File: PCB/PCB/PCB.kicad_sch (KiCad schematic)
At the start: 30 parts, among them J1 AudioJack Right, J2 USB_B_Micro, J3 AudioJack Left, Q1 BC817, Q2 BC817, Q3 BSS84, U1 ESP32-S3-WROOM-1, U2 CP2102N-Axx-xQFN28, U3 NCP1117-3.3_SOT223, U4 UDA1334ATS, U5 PAM8403D

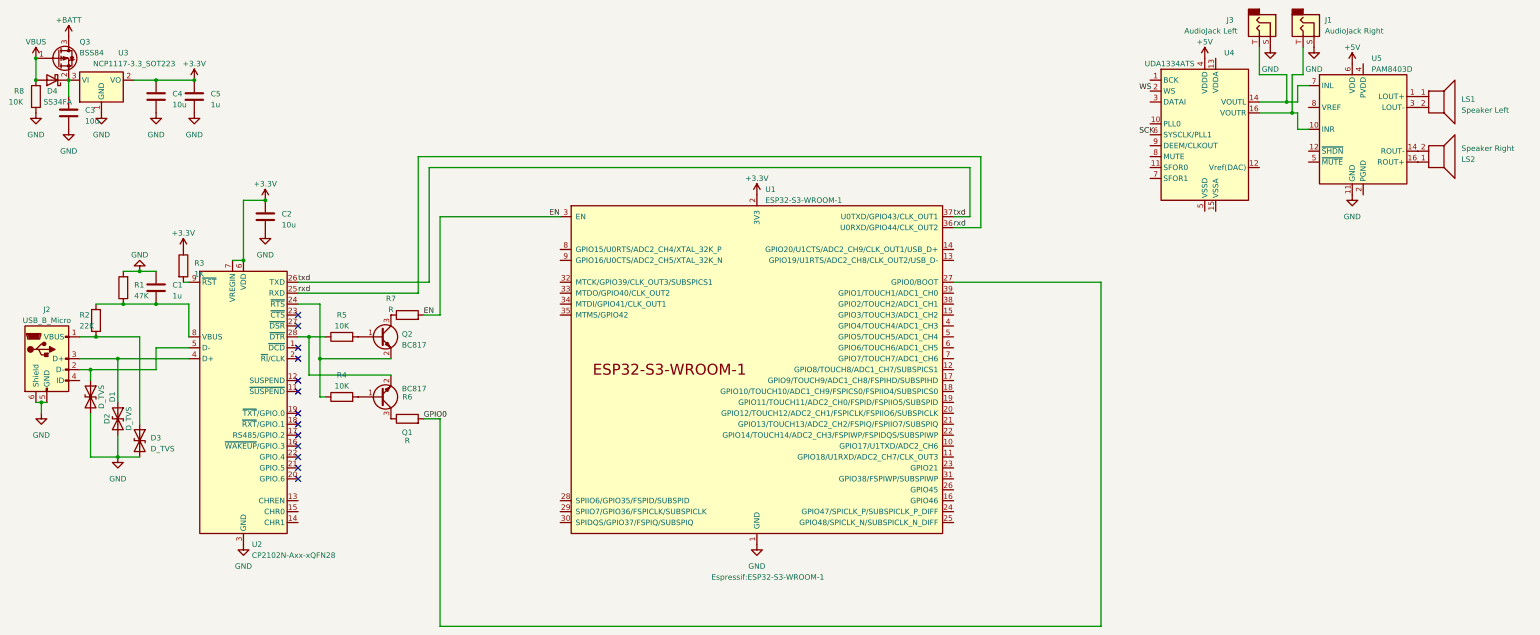
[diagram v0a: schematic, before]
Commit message: edit Vorlesung
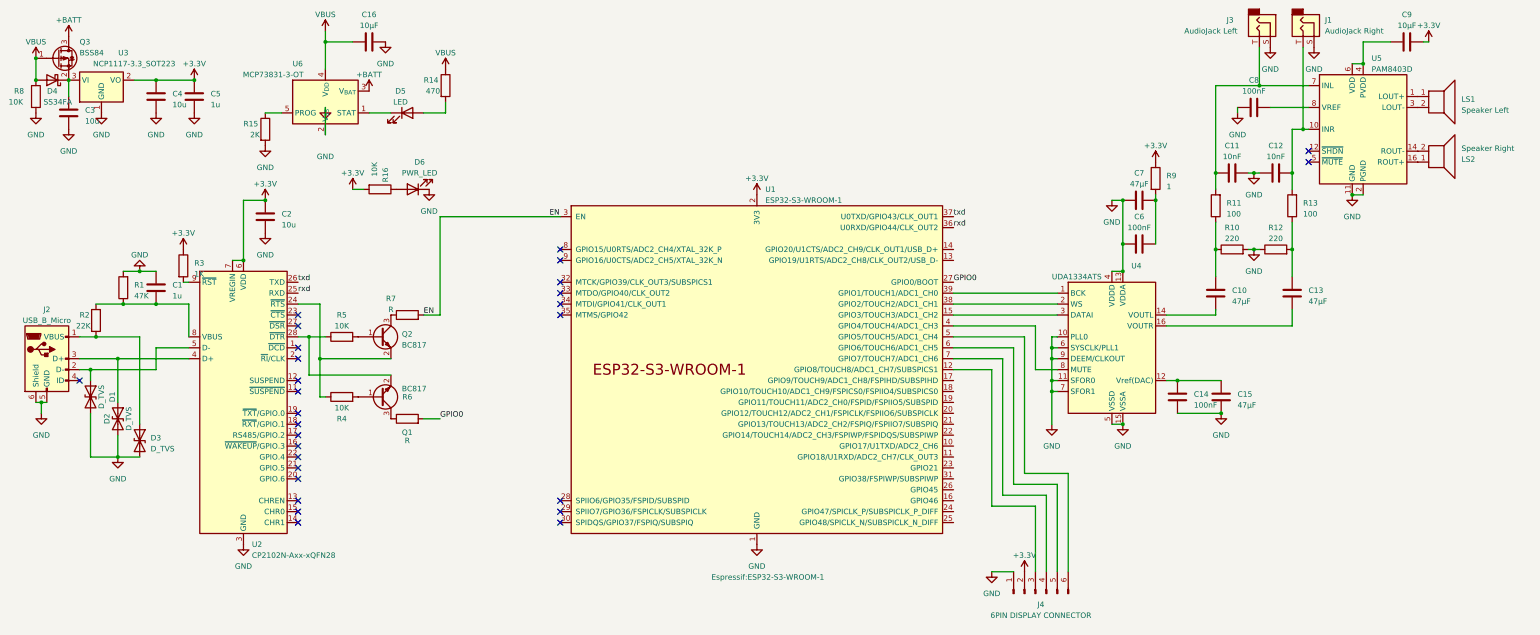
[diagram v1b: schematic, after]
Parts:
- added C10, C13, C15, C7: 47µF, symbol Device:C
- added C11, C12: 10nF, symbol Device:C
- added C14, C6, C8: 100nF, symbol Device:C
- added C16, C9: 10µF, symbol Device:C
- added D5: LED, symbol Device:LED
- added D6: PWR_LED, symbol Device:LED
- added J4: 6PIN DISPLAY CONNECTOR, symbol Connector:Conn_01x06_Pin
- added R10, R12: 220, symbol Device:R
- added R11, R13: 100, symbol Device:R
- added R14: 470, symbol Device:R
- added R15: 2K, symbol Device:R
- added R16: 10K, symbol Device:R
- added R9: 1, symbol Device:R
- added U6: MCP73831-3-OT, Package_TO_SOT_SMD:SOT-23-5, symbol Battery_Management:MCP73831-3-OT
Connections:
- net +3.3V: now also C9.2, J4.2 (Pin_2), R16.2, R9.1
- net +BATT: now also U6.3 (V_{BAT})
- net GND: now also U4.10 (PLL0), U4.11 (SFOR0), U4.13 (VDDA), U4.15 (VSSA), U4.4 (VDDD), U4.5 (VSSD), U4.6 (SYSCLK/PLL1), U4.7 (SFOR1), U4.9 (DEEM/CLKOUT), U5.15 (PGND), U5.2 (PGND), C11.2, C12.1, C14.2, C15.2, C16.2, C6.1, C7.1, C8.1, D6.1 (K), J4.1 (Pin_1), R10.2, R12.1, R15.2, U6.2 (V_{SS})
- net VBUS: now also C16.1, R14.1, U6.4 (V_{DD})
- net at U1.12 (GPIO8/TOUCH8/ADC1_CH7/SUBSPICS1): now also J4.3 (Pin_3)
- net at U1.15 (GPIO3/TOUCH3/ADC1_CH2): now also U4.3 (DATAI)
- net at U1.38 (GPIO2/TOUCH2/ADC1_CH1): now also U4.2 (WS)
- net at U1.39 (GPIO1/TOUCH1/ADC1_CH0): now also U4.1 (BCK)
- net at U1.4 (GPIO4/TOUCH4/ADC1_CH3): now also U4.8 (MUTE)
- net at U1.5 (GPIO5/TOUCH5/ADC1_CH4): now also J4.6 (Pin_6)
- net at U1.6 (GPIO6/TOUCH6/ADC1_CH5): now also J4.5 (Pin_5)
- net at U1.7 (GPIO7/TOUCH7/ADC1_CH6): now also J4.4 (Pin_4)
- net at J1.T, U5.10 (INR): now also C12.2, R13.2; no longer U4.16 (VOUTR)
- net at U5.13 (PVDD), U5.4 (PVDD): now also U5.6 (VDD), C9.1
- net at J3.T, U5.7 (INL): now also C11.1, R11.2; no longer U4.14 (VOUTL)
- net at U5.8 (VREF): now also C8.2
- net at U4.12 (Vref(DAC)): now also C14.1, C15.1
- removed net +5V: U4.4 (VDDD), U5.6 (VDD)
- new net: R15.1, U6.5 (PROG)
- new net: C6.2, C7.2, R9.2
- new net: D6.2 (A), R16.1
- new net: C13.1, U4.16 (VOUTR)
- new net: C13.2, R12.2, R13.1
- new net: C10.1, U4.14 (VOUTL)
- new net: C10.2, R10.1, R11.1
- new net: D5.2 (A), R14.2
- new net: D5.1 (K), U6.1 (STAT)
- no-connect marks 13 -> 28
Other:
- moved on the sheet: U4
